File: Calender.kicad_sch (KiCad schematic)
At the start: 52 parts, among them J1 Conn_01x09, J2 USB_C_Receptacle_USB2.0_16P, J3 Power, J4 Screen-2, SW1 RotaryEncoder_Switch, SW2 SW_Push, SW3 SW_Push, SW4 SW_Push, U1 ATSAMD21G18A-A, U3 MCP73871, U4 AMS1117-3.3, U5 ESP-WROOM-02, U6 NAND

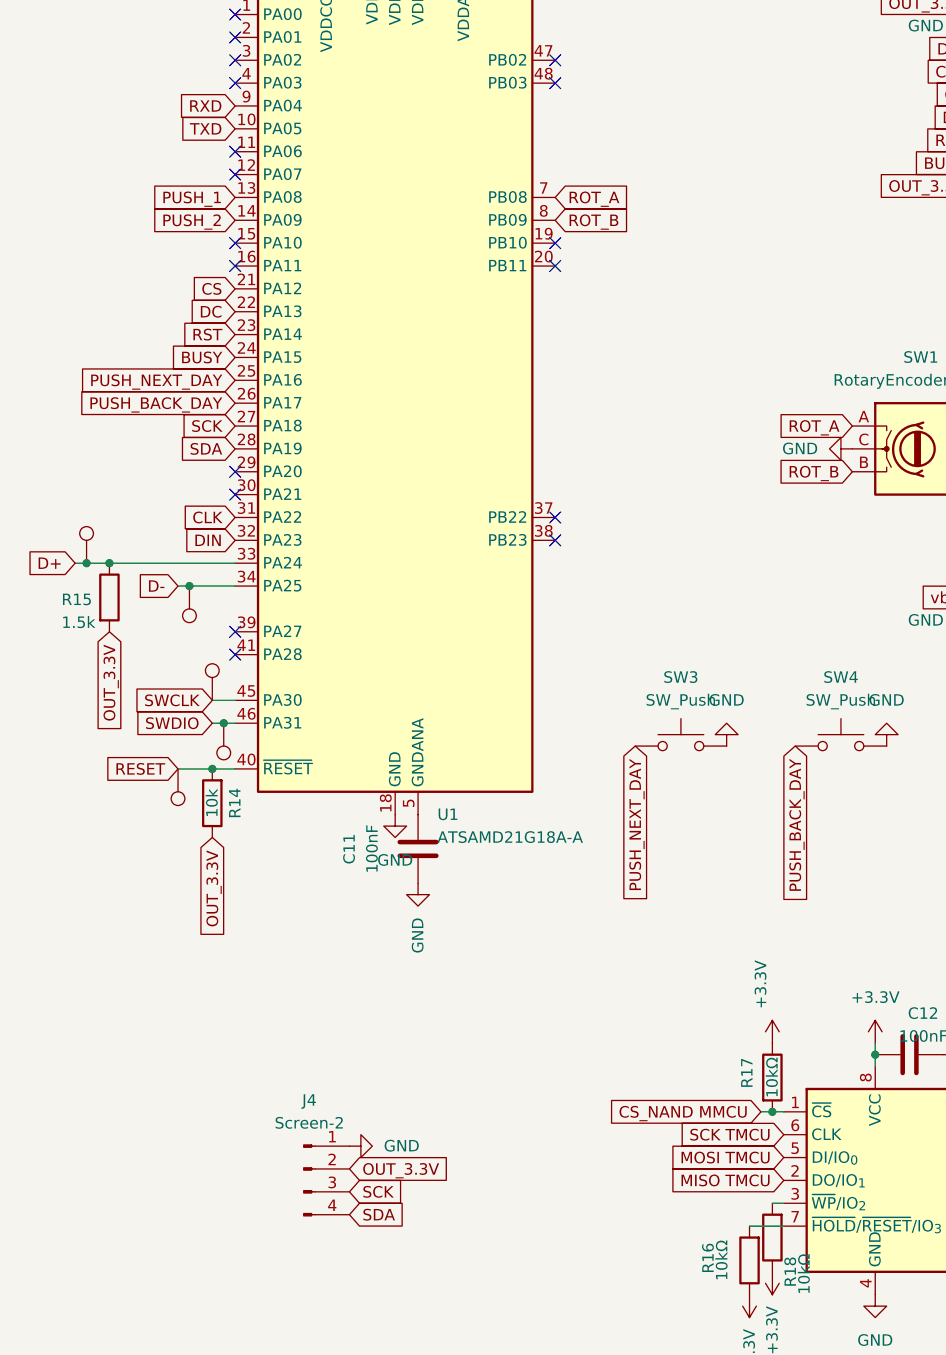
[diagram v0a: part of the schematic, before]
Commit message: Should be finished
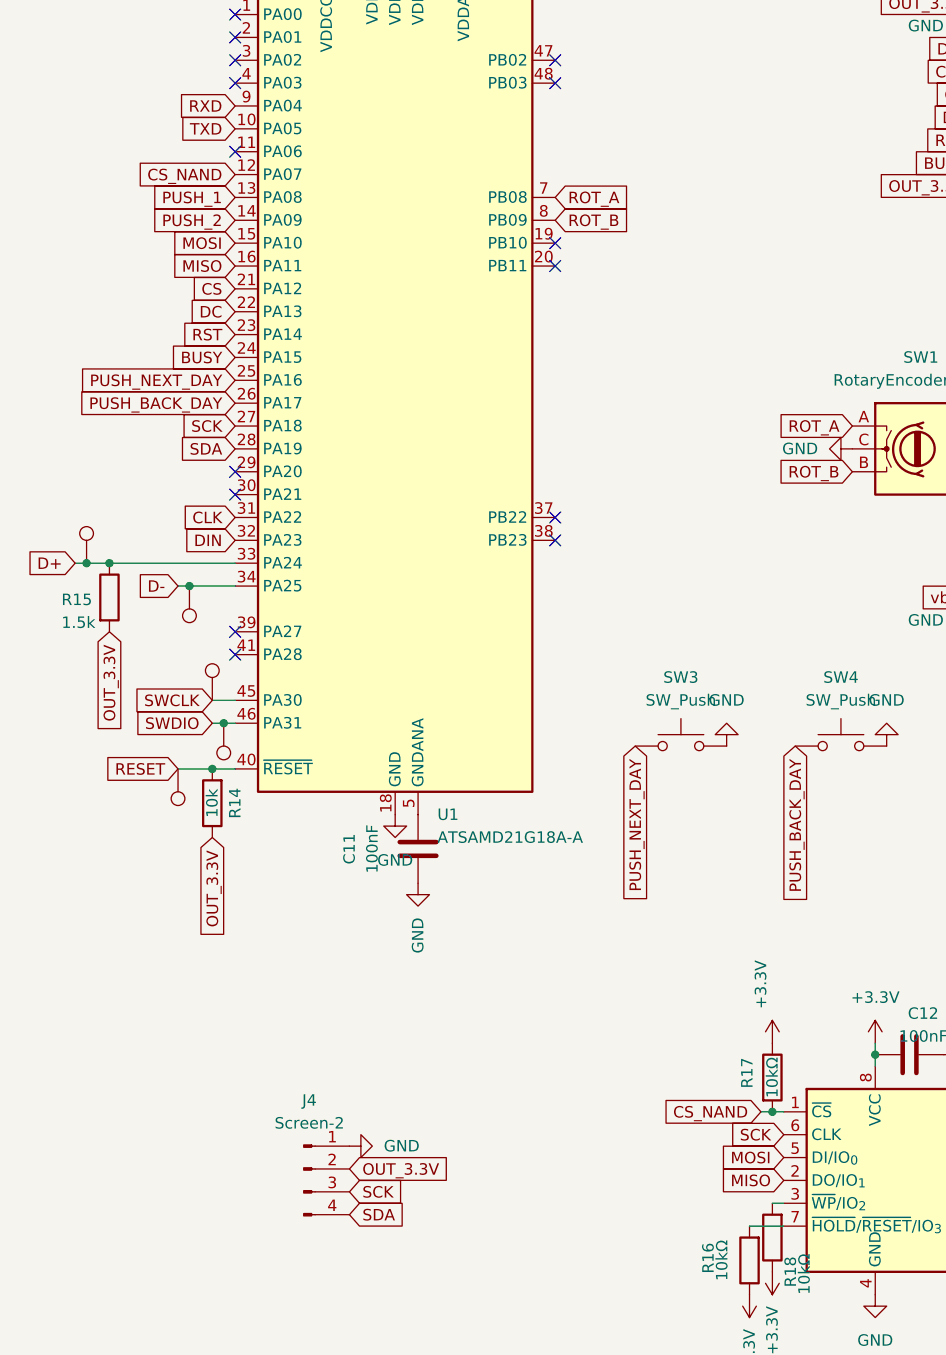
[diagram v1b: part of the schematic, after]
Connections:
- net CS_NAND MMCU is gone; now on net CS_NAND: R17.2, U6.1 (~{CS})
- net MISO TMCU is gone; now on net MISO: U6.2 (DO/IO_{1})
- net MOSI TMCU is gone; now on net MOSI: U6.5 (DI/IO_{0})
- net SCK TMCU is gone; now on net SCK: U6.6 (CLK)
- net CS_NAND: now reaches U1.12 (PA07)
- net MOSI: now reaches U1.15 (PA10)
- net MISO: now reaches U1.16 (PA11)
- no-connect marks 29 -> 26
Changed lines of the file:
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@@
-	)
-	(no_connect
-		(at 43.18 66.04)
 	)
 	(no_connect
@@
 	)
 	(no_connect
-		(at 43.18 63.5)
-	)
-	(no_connect
 		(at 257.81 133.35)
 	)
@@
 	)
 	(no_connect
-		(at 43.18 55.88)
-	)
-	(no_connect
 		(at 257.81 143.51)
 	)
@@
 		)
 	)
-	(global_label "CS_NAND MMCU"
+	(global_label "CS_NAND"
 		(shape input)
 		(at 101.6 160.02 180)
@@
 		)
 		(property "Intersheetrefs" "${INTERSHEET_REFS}"
-			(at 83.6772 160.02 0)
+			(at 90.1481 160.02 0)
 			(effects
 				(font
@@
 		)
 	)
+	(global_label "CS_NAND"
+		(shape input)
+		(at 43.18 55.88 180)
+		(fields_autoplaced yes)
+		(effects
+			(font
+				(size 1.27 1.27)
+			)
+			(justify right)
+		)
+		(property "Intersheetrefs" "${INTERSHEET_REFS}"
+			(at 31.7281 55.88 0)
+			(effects
+				(font
+					(size 1.27 1.27)
+				)
+				(justify right)
+				(hide yes)
+			)
+		)
+	)
 	(global_label "PUSH_1"
 		(shape input)
@@
 		)
 	)
-	(global_label "MOSI TMCU"
+	(global_label "MOSI"
 		(shape input)
 		(at 104.14 165.1 180)
@@
 		)
 		(property "Intersheetrefs" "${INTERSHEET_REFS}"
-			(at 90.5715 165.1 0)
+			(at 96.5586 165.1 0)
 			(effects
 				(font
@@
 		)
 	)
-	(global_label "MISO TMCU"
+	(global_label "MISO"
 		(shape input)
 		(at 104.14 167.64 180)
@@
 		)
 		(property "Intersheetrefs" "${INTERSHEET_REFS}"
-			(at 90.5715 167.64 0)
-			(effects
-				(font
-					(size 1.27 1.27)
-				)
-				(justify right)
-				(hide yes)
-			)
-		)
-	)
-	(global_label "SCK TMCU"
+			(at 96.5586 167.64 0)
+			(effects
+				(font
+					(size 1.27 1.27)
+				)
+				(justify right)
+				(hide yes)
+			)
+		)
+	)
+	(global_label "SCK"
 		(shape input)
 		(at 104.14 162.56 180)
@@
 		)
 		(property "Intersheetrefs" "${INTERSHEET_REFS}"
-			(at 91.4182 162.56 0)
+			(at 97.4053 162.56 0)
 			(effects
 				(font
@@
 		)
 	)
+	(global_label "MOSI"
+		(shape input)
+		(at 43.18 63.5 180)
+		(fields_autoplaced yes)
+		(effects
+			(font
+				(size 1.27 1.27)
+			)
+			(justify right)
+		)
+		(property "Intersheetrefs" "${INTERSHEET_REFS}"
+			(at 35.5986 63.5 0)
+			(effects
+				(font
+					(size 1.27 1.27)
+				)
+				(justify right)
+				(hide yes)
+			)
+		)
+	)
 	(global_label "CLK"
 		(shape input)
@@
 				(hide yes)
 			)
+		)
+	)
+	(global_label "MISO"
+		(shape input)
+		(at 43.18 66.04 180)
+		(fields_autoplaced yes)
+		(effects
+			(font
+				(size 1.27 1.27)
+			)
+			(justify right)
+		)
+		(property "Intersheetrefs" "${INTERSHEET_REFS}"
+			(at 35.5986 66.04 0)
+			(effects
+				(font
+					(size 1.27 1.27)
+				)
+				(justify right)
+				(hide yes)
+			)
